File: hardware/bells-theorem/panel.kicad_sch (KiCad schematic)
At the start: 79 parts, among them J10 D, J11 C, J12 DA, J13 CD, J14 DAB, J15 CDA, J16 A, J17 B, J18 AB, J19 BC, J20 ABC, J21 BCD, J22 left, J23 right, J4 IN, J5 CVA, J6 CVB, J7 CVC, J8 CVD, J9 ABCD, Q11 2N3904, Q2 2N3904, Q5 2N3904, Q8 2N3904

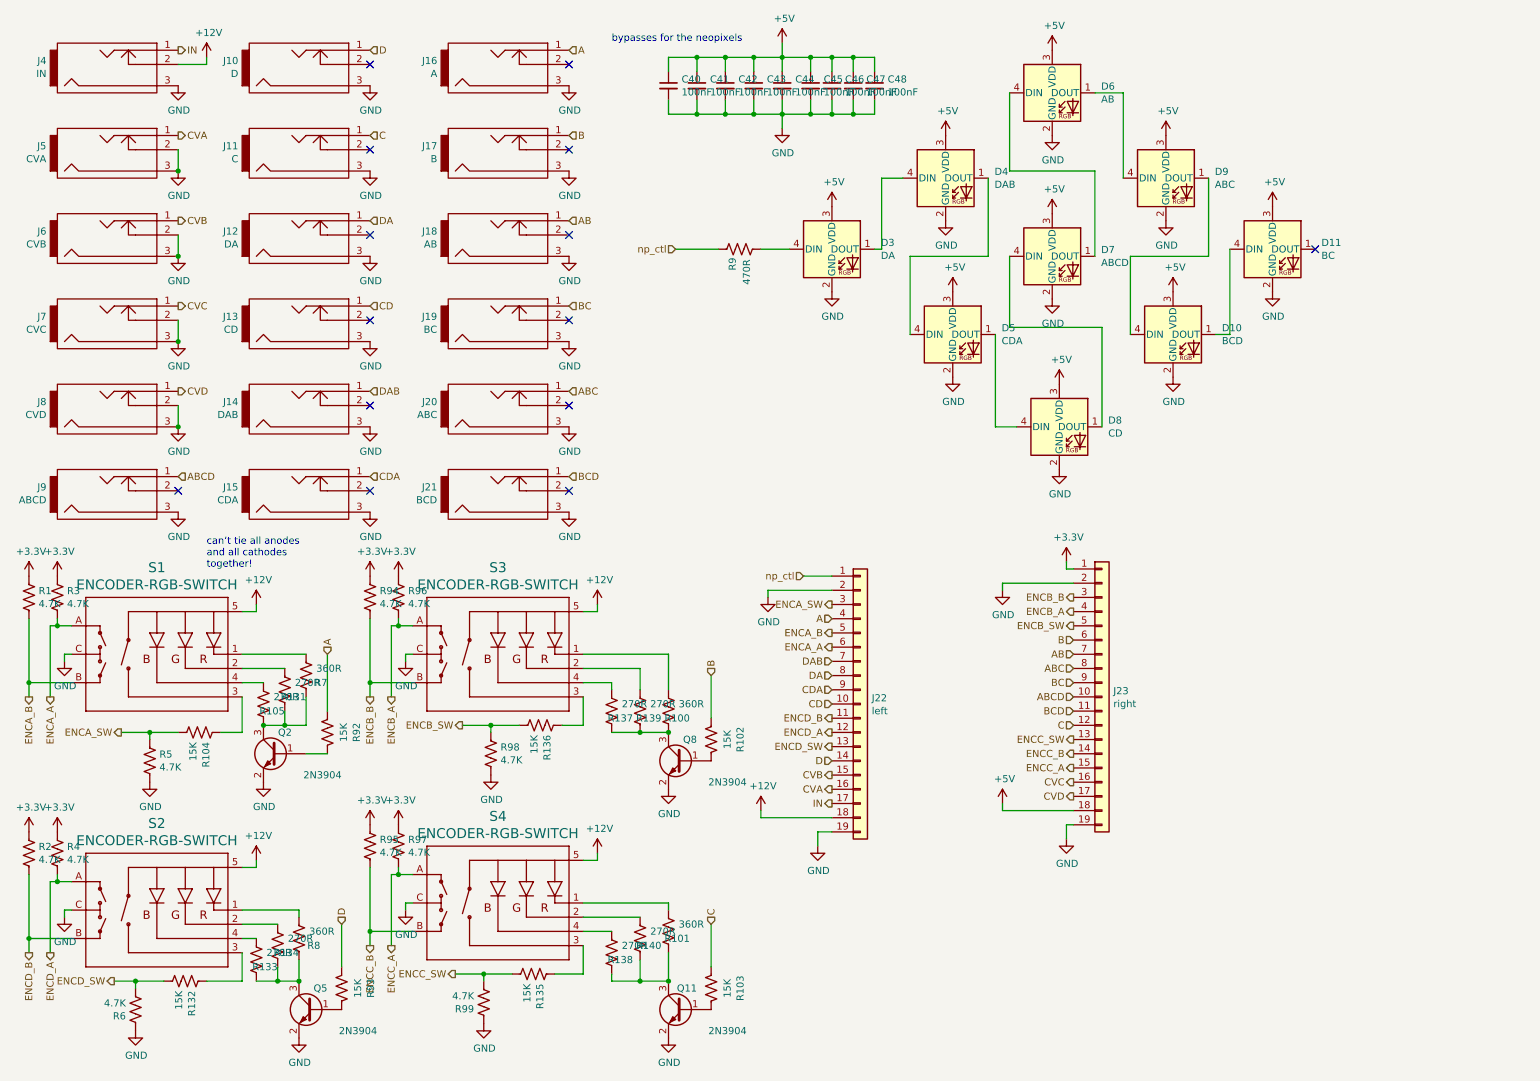
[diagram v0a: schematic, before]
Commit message: last hardware / software updates
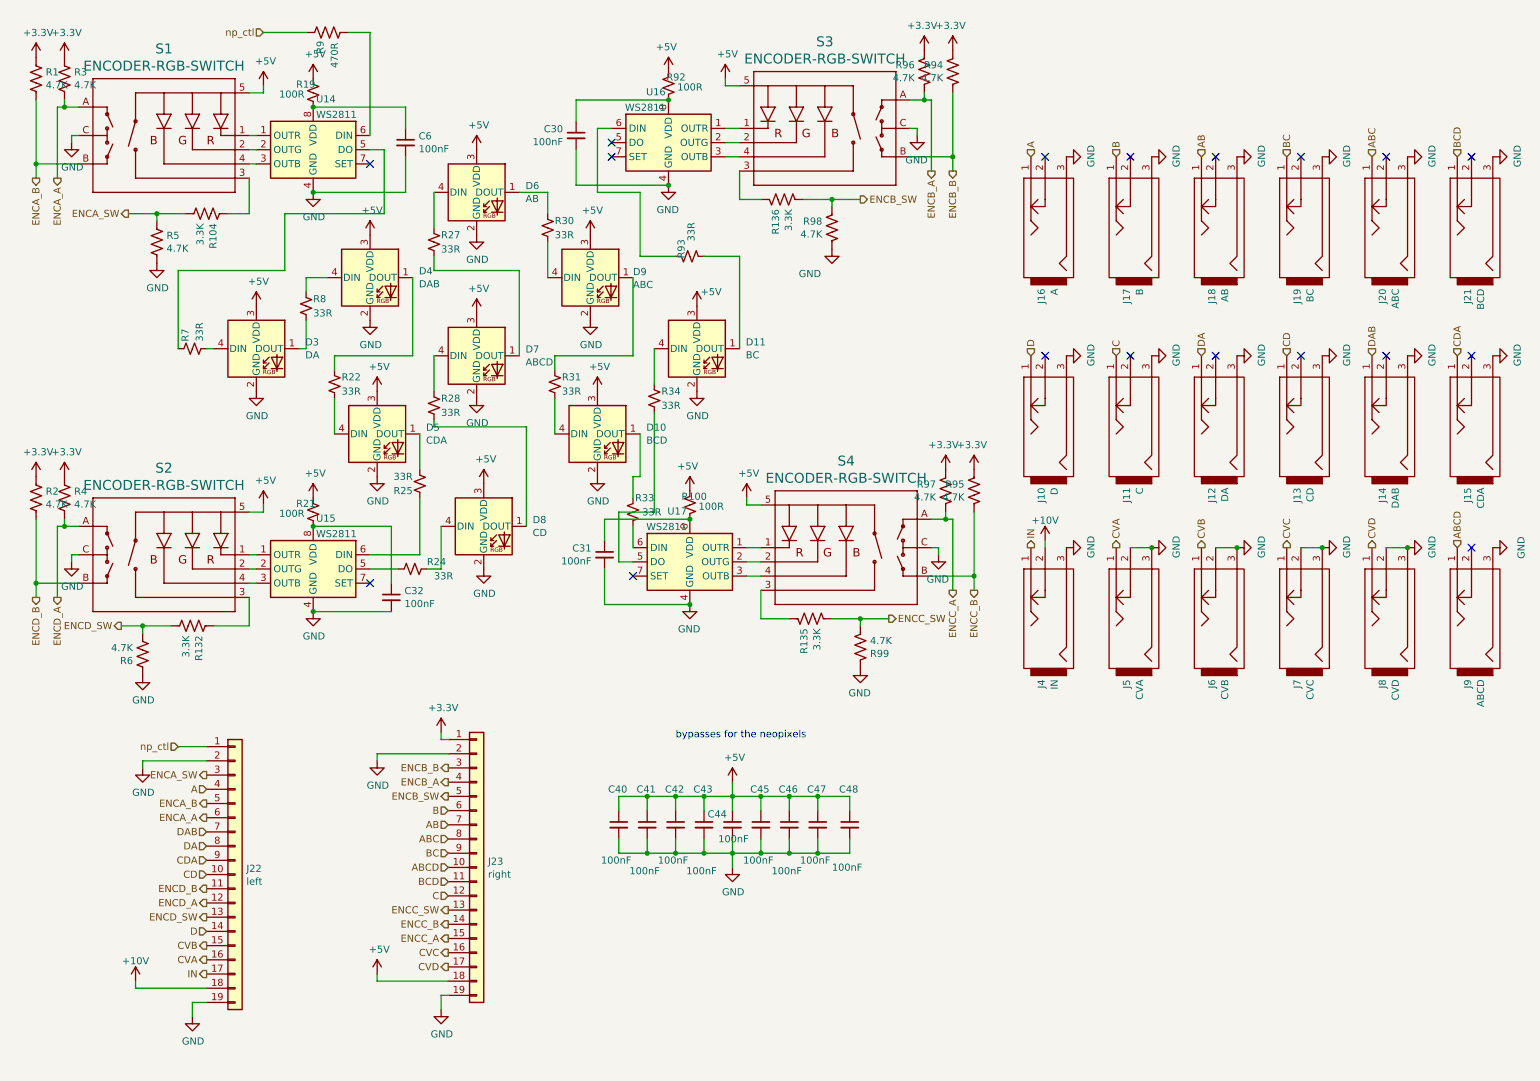
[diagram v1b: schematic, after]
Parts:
- removed Q11, Q2, Q5, Q8: 2N3904, Package_TO_SOT_SMD:SOT-23_Handsoldering, symbol Device:Q_NPN_BEC
- removed R100, R101, R7, R8: 360R, Resistor_SMD:R_0805_2012Metric_Pad1.20x1.40mm_HandSolder, symbol Device:R_US
- removed R102, R103, R92, R93: 15K, Resistor_SMD:R_0805_2012Metric_Pad1.20x1.40mm_HandSolder, symbol Device:R_US
- removed R105, R131, R133, R134, R137, R138, R139, R140: 270R, Resistor_SMD:R_0805_2012Metric_Pad1.20x1.40mm_HandSolder, symbol Device:R_US
- added C30, C31, C32, C6: 100nF, Capacitor_SMD:C_0805_2012Metric_Pad1.18x1.45mm_HandSolder, symbol Device:C_Small
- added R100, R19, R21, R92: 100R, Resistor_SMD:R_0805_2012Metric_Pad1.20x1.40mm_HandSolder, symbol Device:R_Small_US
- added R22, R24, R25, R27, R28, R30, R31, R33, R34, R7, R8, R93: 33R, Resistor_SMD:R_0805_2012Metric_Pad1.20x1.40mm_HandSolder, symbol Device:R_Small_US
- added U14, U15, U16, U17: WS2811, Package_SO:SOIC-8_3.9x4.9mm_P1.27mm, symbol Driver_LED:WS2811
- R104, R132, R135, R136: value 15K -> 3.3K
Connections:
- net +5V: now also S1.5 (+), S2.5 (+), S3.5 (+), S4.5 (+), R100.1, R19.1, R21.1, R92.1
- net GND: now also C30.2, C31.2, C32.2, C6.2, U14.4 (GND), U15.4 (GND), U16.4 (GND), U17.4 (GND)
- net at S1.2 (-G): now also U14.2 (OUTG)
- net at S1.4 (-B): now also U14.3 (OUTB)
- net at S1.1 (-R): now also U14.1 (OUTR)
- net at S3.1 (-R): now also U16.1 (OUTR)
- net at S3.2 (-G): now also U16.2 (OUTG)
- net at S3.4 (-B): now also U16.3 (OUTB)
- net at S4.1 (-R): now also U17.1 (OUTR)
- net at S4.2 (-G): now also U17.2 (OUTG)
- net at S4.4 (-B): now also U17.3 (OUTB)
- net at S2.1 (-R): now also U15.1 (OUTR)
- net at S2.2 (-G): now also U15.2 (OUTG)
- net at S2.4 (-B): now also U15.3 (OUTB)
- net at D6.1 (DOUT): now also R30.1; no longer D9.4 (DIN)
- net at D6.4 (DIN): now also R27.1; no longer D7.1 (DOUT)
- net at D7.4 (DIN): now also R28.1; no longer D8.1 (DOUT)
- net at D8.4 (DIN): now also R24.1; no longer D5.1 (DOUT)
- net at D4.1 (DOUT): now also R22.1; no longer D5.4 (DIN)
- net at D4.4 (DIN): now also R8.1; no longer D3.1 (DOUT)
- net at D3.4 (DIN): now also R7.2; no longer R9.2
- net at D9.1 (DOUT): now also R31.1; no longer D10.4 (DIN)
- net at D10.1 (DOUT): now also R33.1; no longer D11.4 (DIN)
- net at D11.1 (DOUT): now also R93.2
- removed net +12V: J22.18 (Pin_18), J4.2, S1.5 (+), S2.5 (+), S3.5 (+), S4.5 (+)
- new net: D7.1 (DOUT), R27.2
- new net: D8.1 (DOUT), R28.2
- new net: D5.1 (DOUT), R25.2
- new net: D5.4 (DIN), R22.2
- new net: D3.1 (DOUT), R8.2
- new net: D9.4 (DIN), R30.2
- new net: D10.4 (DIN), R31.2
- new net: D11.4 (DIN), R34.1
- new net: R9.2, U14.6 (DIN)
- new net: R93.1, U16.6 (DIN)
- new net: C30.1, R92.2, U16.8 (VDD)
- new net: C31.1, R100.2, U17.8 (VDD)
- new net: R7.1, U14.5 (DO)
- new net: C6.1, R19.2, U14.8 (VDD)
- new net: R24.2, U15.5 (DO)
- new net: R25.1, U15.6 (DIN)
- new net: C32.1, R21.2, U15.8 (VDD)
- new net: R34.2, U17.5 (DO)
- new net: R33.2, U17.6 (DIN)
- new net +10V: J22.18 (Pin_18), J4.2
- no-connect marks 14 -> 18
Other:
- note removed: "can’t tie all anodes and all cathodes together!"
- moved on the sheet: C40, C41, C42, C43, C44, C45, C46, C47, C48, D10, D11, D3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
